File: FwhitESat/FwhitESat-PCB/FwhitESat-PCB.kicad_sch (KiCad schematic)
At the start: 5 parts, among them U1 3Ter-Reg-3.3Vout, U2 DCDC-5Vout

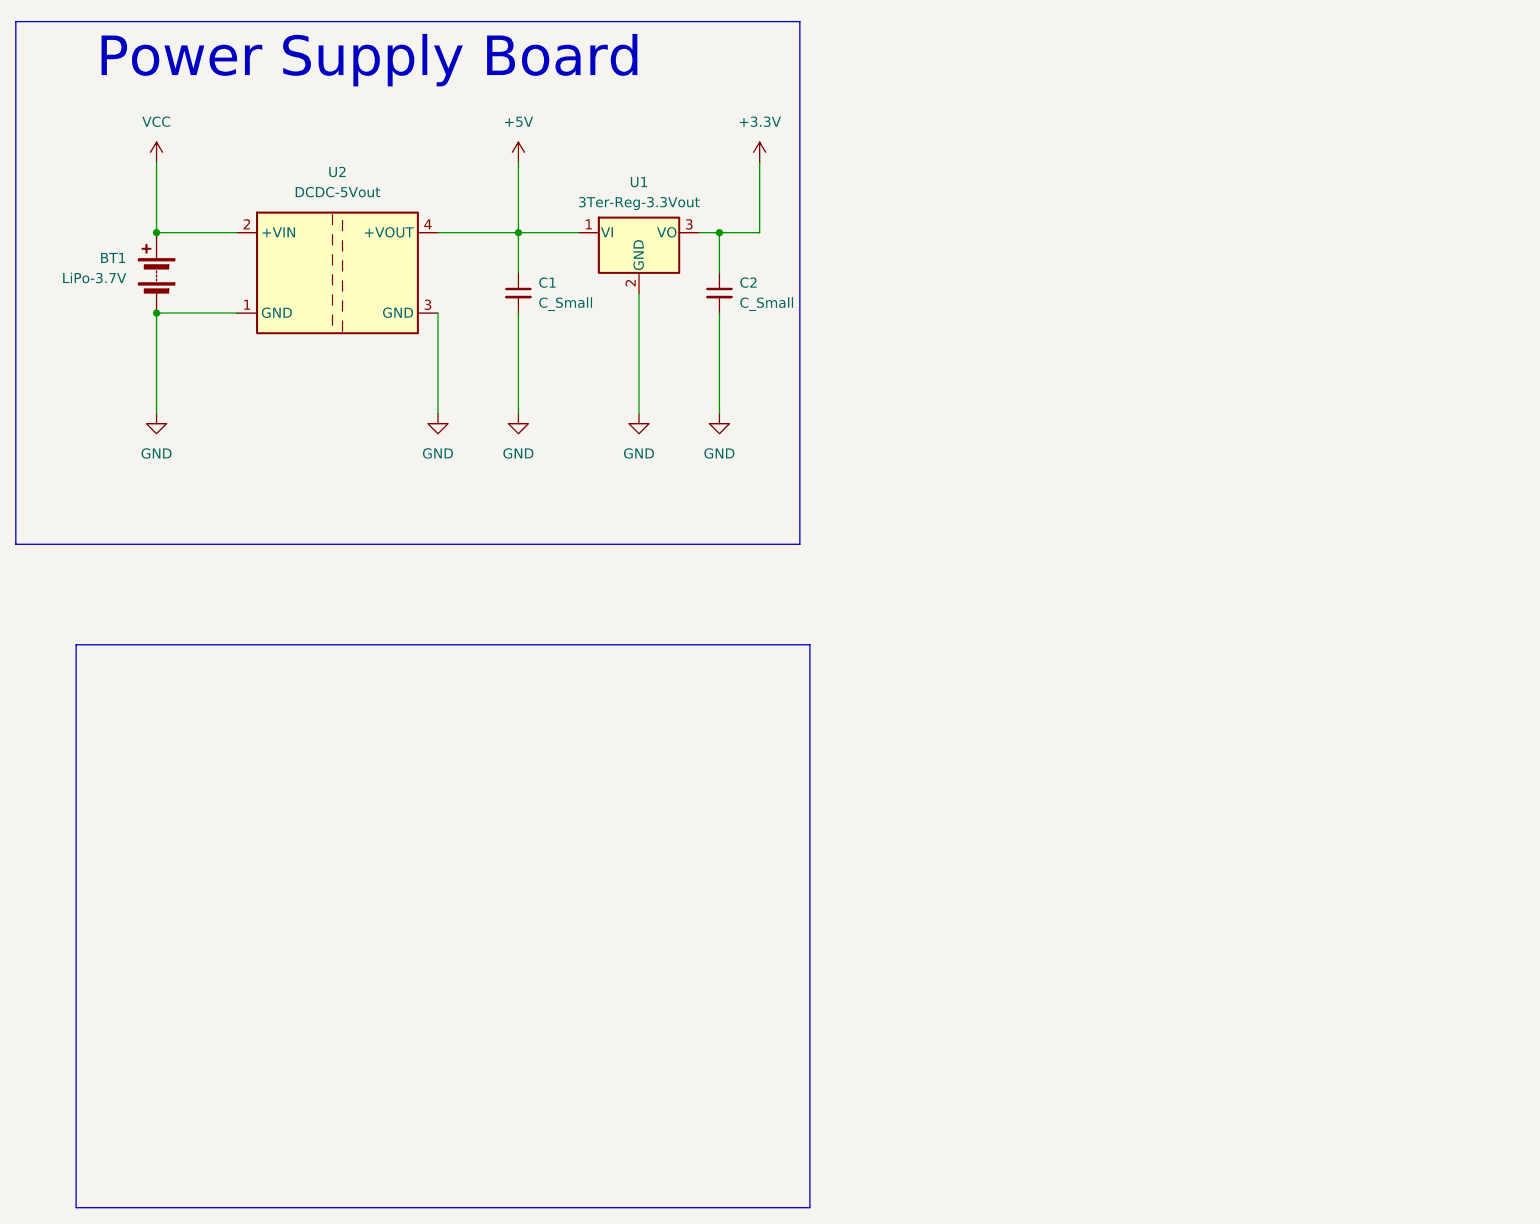
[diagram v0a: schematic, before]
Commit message: fix FwhitESat/FwhitESat-PCB
Each module was divided into layers.
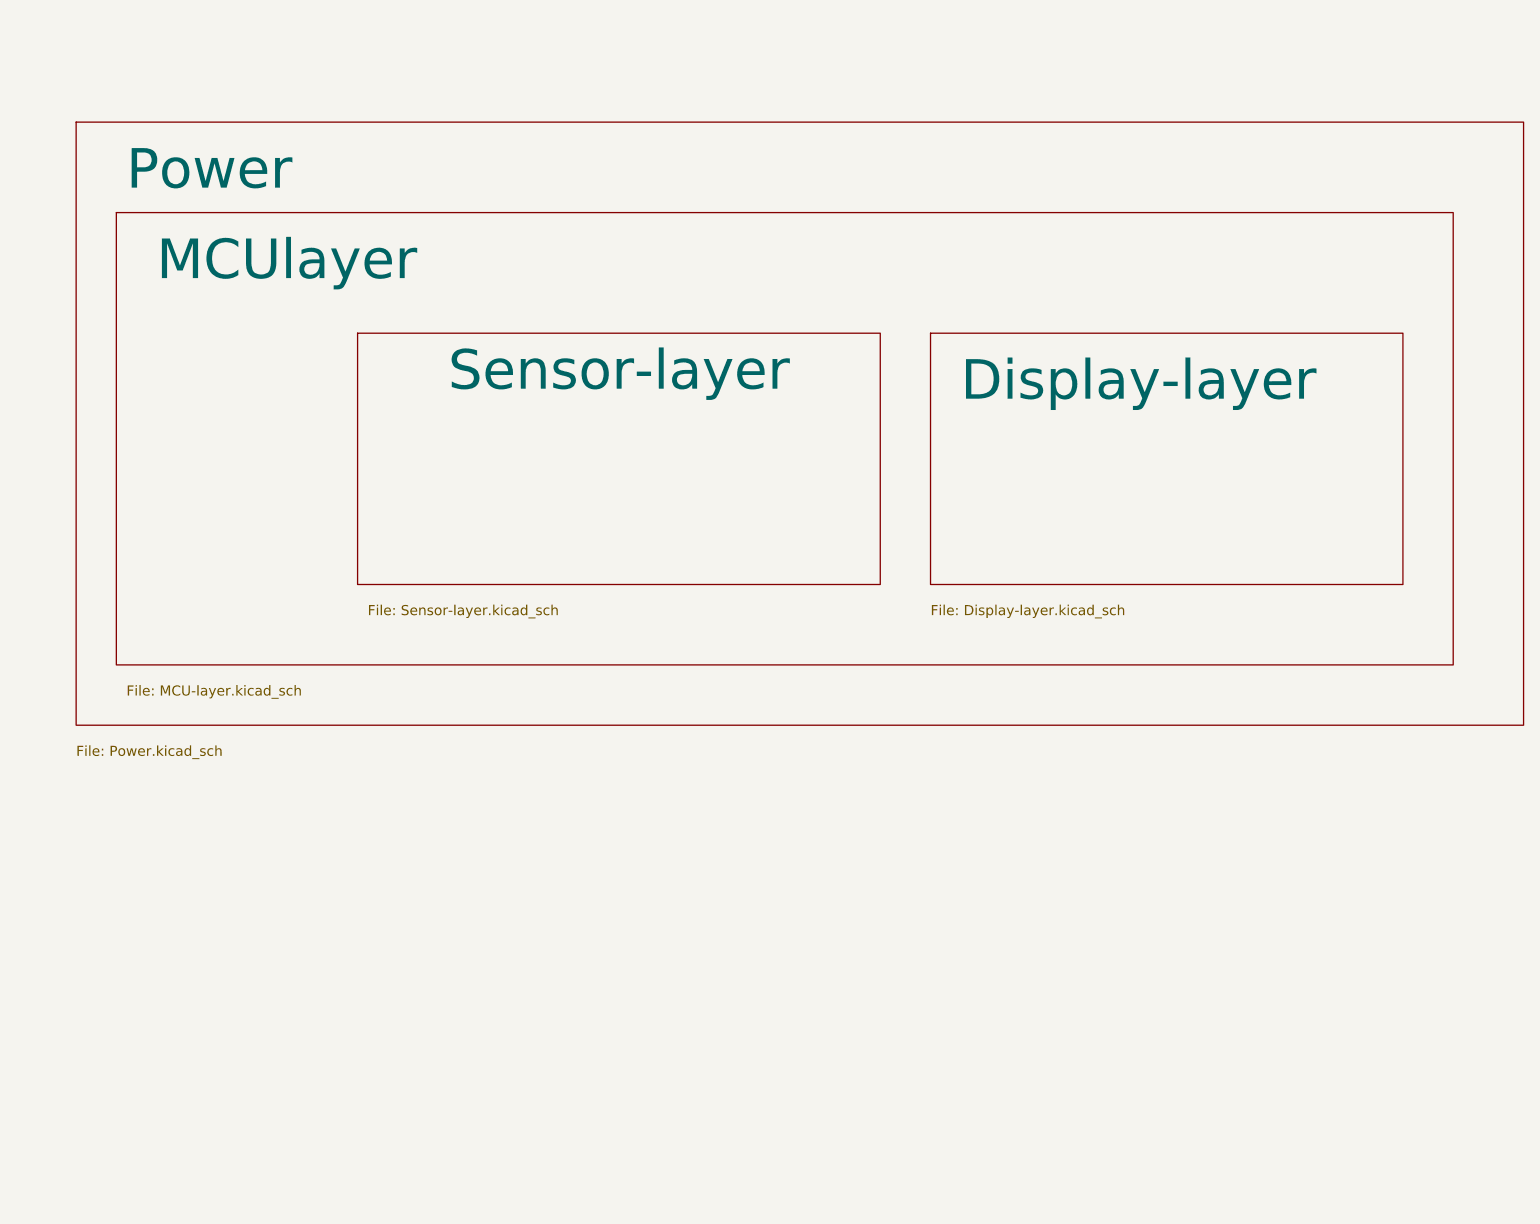
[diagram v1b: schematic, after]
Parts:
- removed BT1: LiPo-3.7V, symbol 01-FwhitESat-Local_Library:Battery
- removed C1, C2: C_Small, symbol Device:C_Small
- removed U1: 3Ter-Reg-3.3Vout, Package_TO_SOT_THT:TO-220-3_Vertical, symbol 01-FwhitESat-Local_Library:3Ter-Reg-3.3Vout
- removed U2: DCDC-5Vout, Converter_DCDC:Converter_DCDC_Murata_CRE1xxxxxx3C_THT, symbol 01-FwhitESat-Local_Library:DCDC-5Vout
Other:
- added sheet Display-layer (Display-layer.kicad_sch)
- added sheet MCUlayer (MCU-layer.kicad_sch)
- added sheet Power (Power.kicad_sch)
- added sheet Sensor-layer (Sensor-layer.kicad_sch)
- note removed: "Power Supply Board"
